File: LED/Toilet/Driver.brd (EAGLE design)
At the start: 32.7 x 39 mm, 19 parts, among them IC1 HV9910BNG

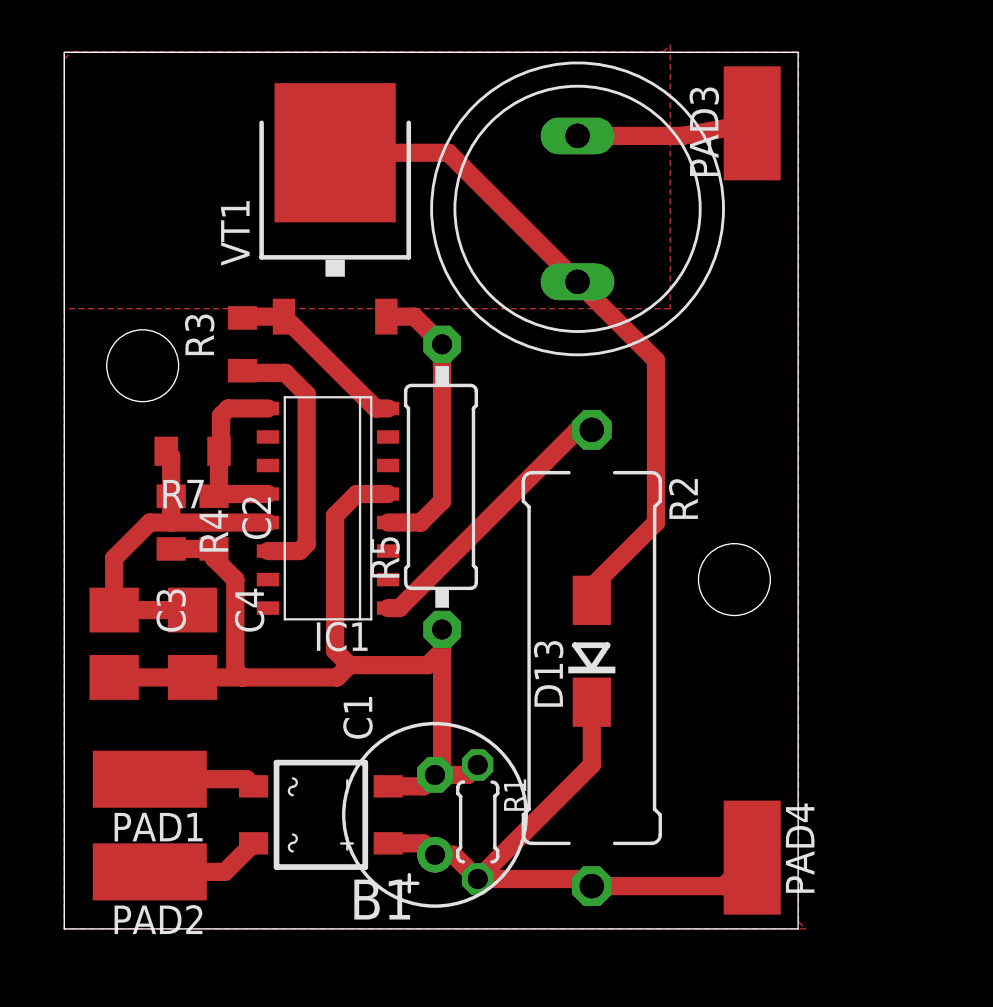
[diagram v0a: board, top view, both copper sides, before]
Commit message: Что-то изменилось
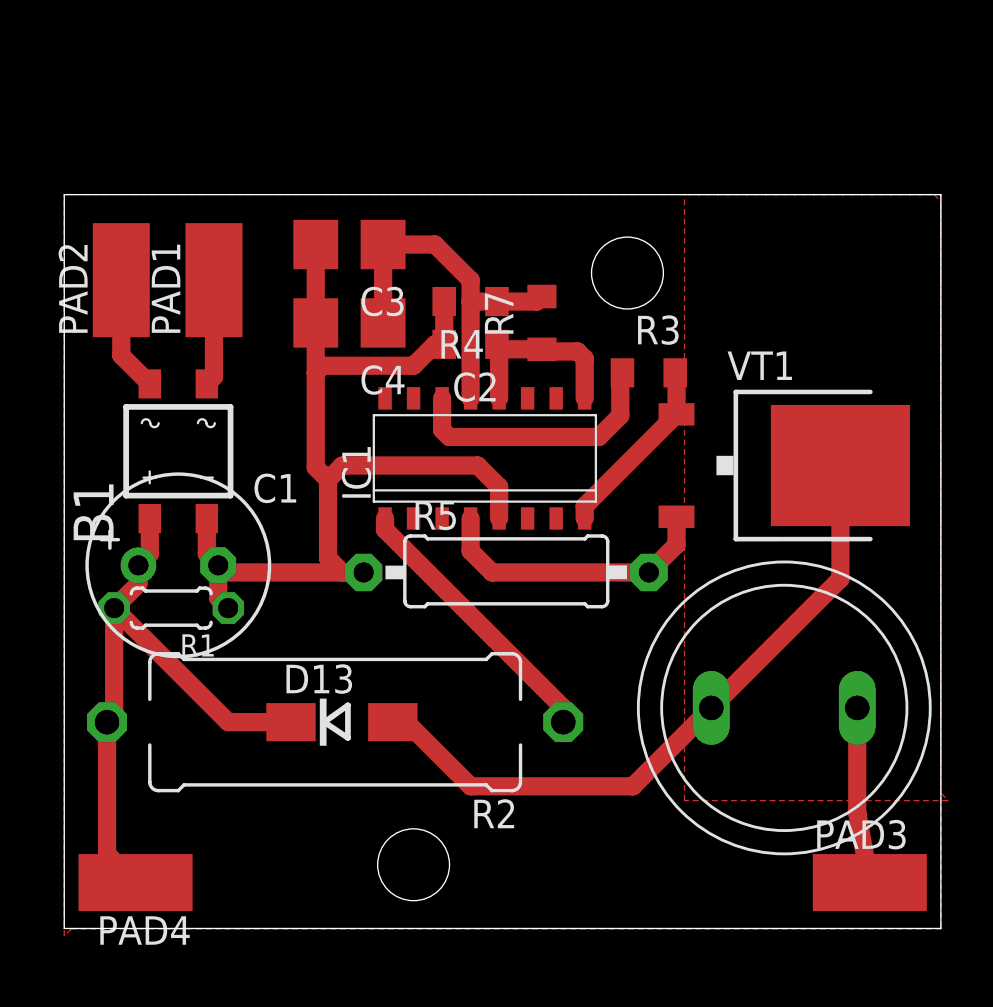
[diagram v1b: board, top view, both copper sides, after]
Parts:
- R3: value 91K -> 75K
- moved PAD3 34.2 mm to (35.9, 2.06), turned to 270 degrees
- moved PAD4 27.5 mm to (3.17, 2.06), turned to 90 degrees
- moved PAD2 26.4 mm to (2.54, 28.9), turned to 0 degrees
- moved L1 24.1 mm to (32.1, 9.84), turned to 180 degrees
- moved VT1 23.0 mm to (32.1, 20.6), turned to 270 degrees
- moved PAD1 22.4 mm to (6.67, 28.9), turned to 0 degrees
- moved C3 20.6 mm to (12.7, 30.5), turned to 180 degrees
- moved R3 18.1 mm to (26.0, 24.8), turned to 0 degrees
- moved B1 17.4 mm to (5.08, 21.3), turned to 0 degrees
- moved R1 16.6 mm to (4.76, 14.3), turned to 180 degrees
- moved R4 16.6 mm to (18.1, 27.9), turned to 180 degrees
- moved R7 16.6 mm to (21.3, 27.0), turned to 90 degrees
- moved C1 15.9 mm to (5.08, 16.2), turned to 0 degrees
- moved C4 15.9 mm to (12.7, 27.0), turned to 180 degrees
- moved C2 13.9 mm to (18.1, 26.0), turned to 180 degrees
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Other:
- board size 32.7 x 39 mm -> 39 x 32.7 mm
